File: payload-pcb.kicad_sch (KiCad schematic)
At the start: 4 parts

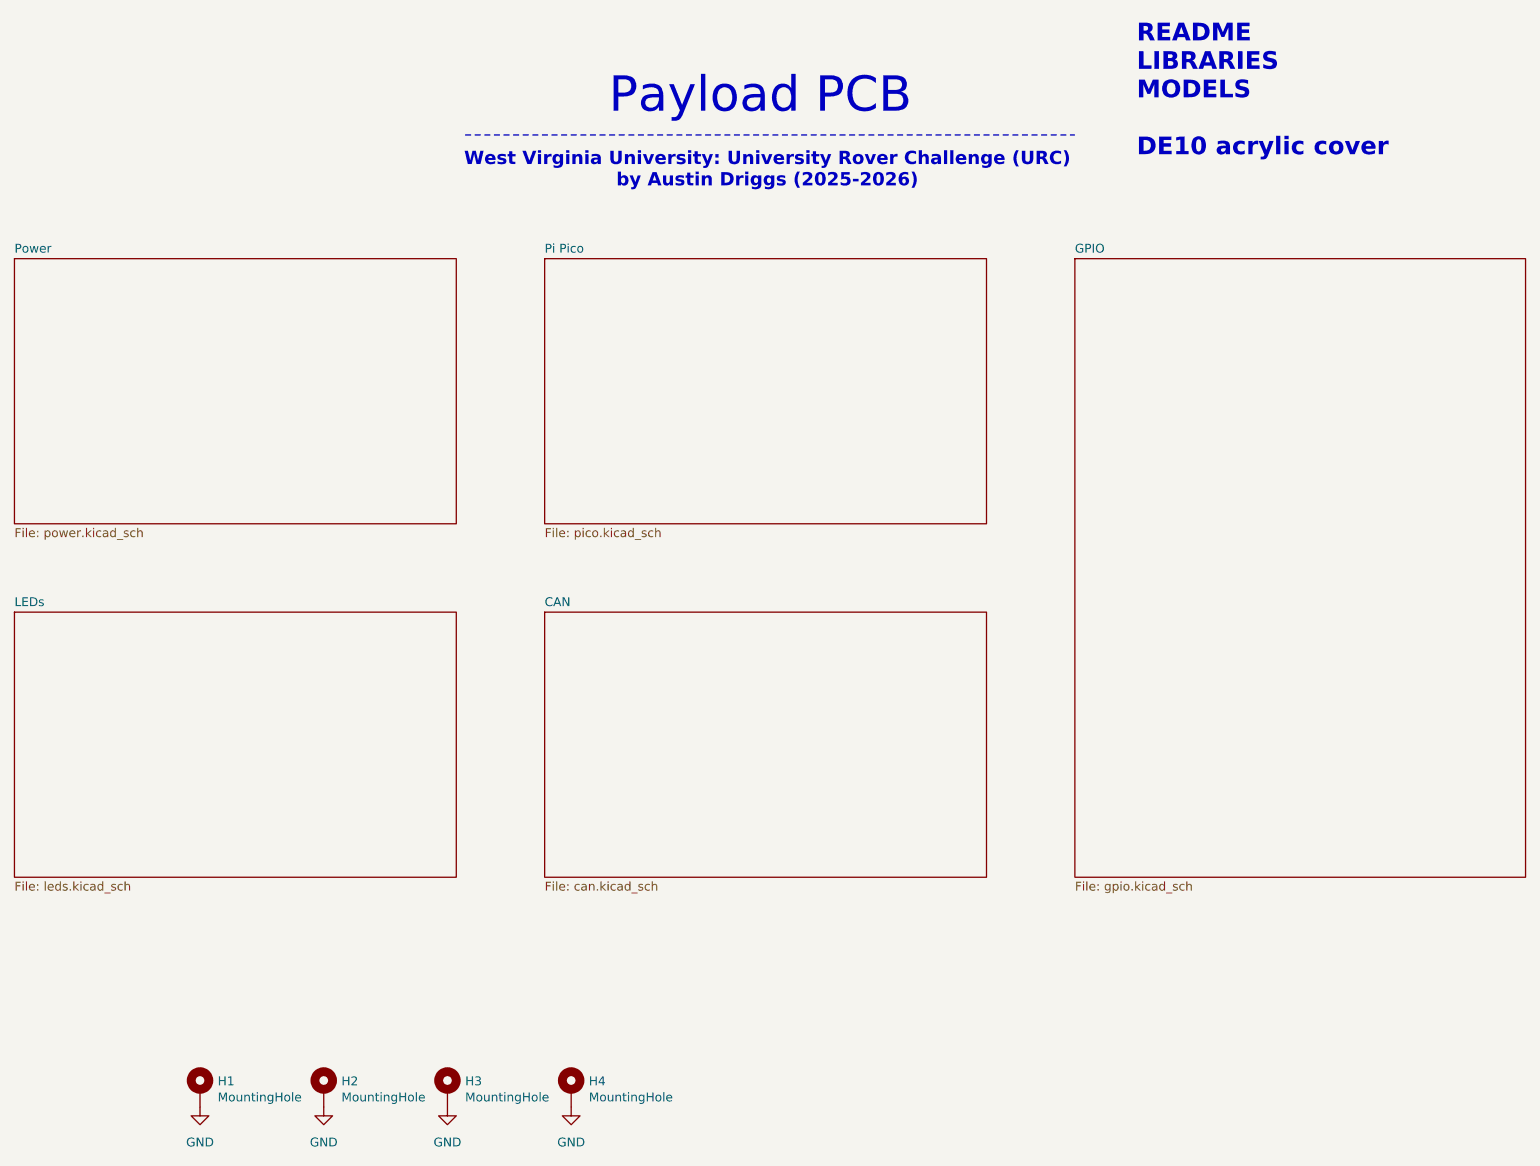
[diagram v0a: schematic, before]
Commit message: major rework again after the meeting
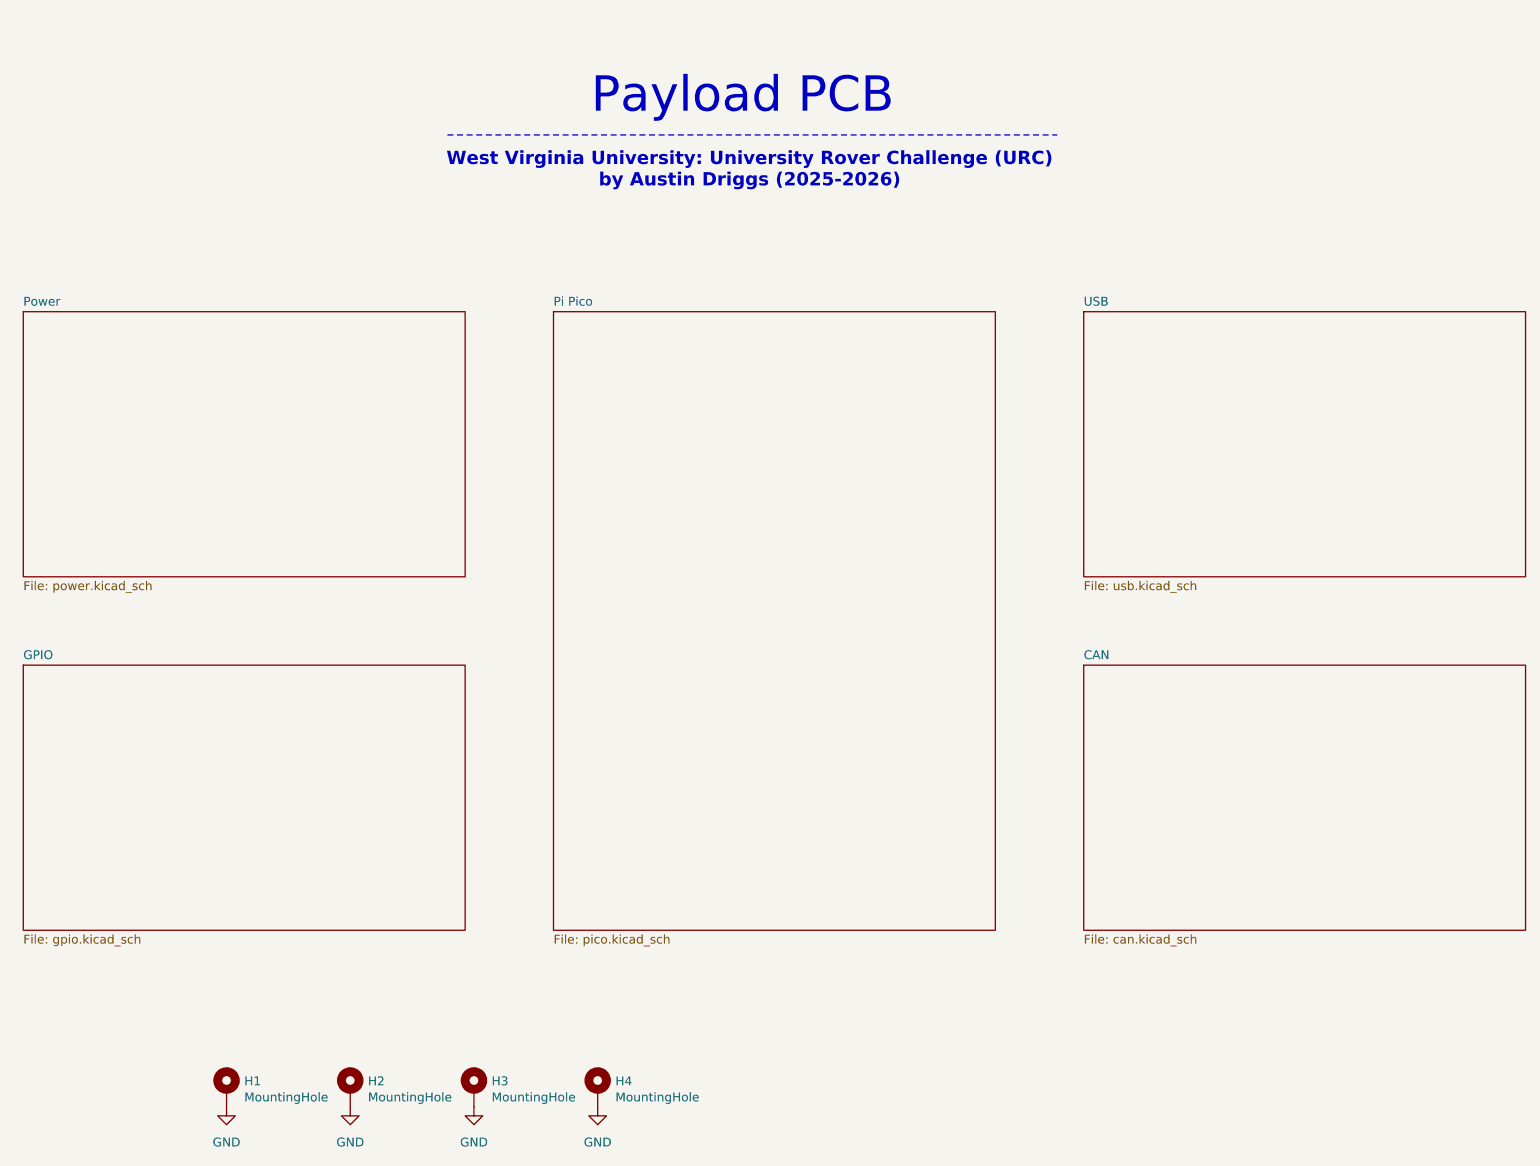
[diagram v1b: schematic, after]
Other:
- removed sheet LEDs
- added sheet USB (usb.kicad_sch)
- note removed: "README LIBRARIES MODELS DE10 acrylic cover"
- moved on the sheet: H1, H2, H3, H4
